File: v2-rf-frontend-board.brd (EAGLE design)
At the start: 89.7 x 43.9 mm, 134 parts, among them J1 1.27MM-SWD-CONNECTOR, J3 ROCKETNET-CONNECTOR-16M, Q1 NTR4101P, T1 ALT4532, T2 ALT4532, U1 MAX2769, U10 LMZ12001, U3 LAN8710A-EZC, U4 7Q-16.368MBG-T, U5 XC2401, U6 MAX8510EXK29+T, U7 MAX8510EXK29+T, U8 STM32F4V, X1 25 MHz, X2 BU-SMA-H

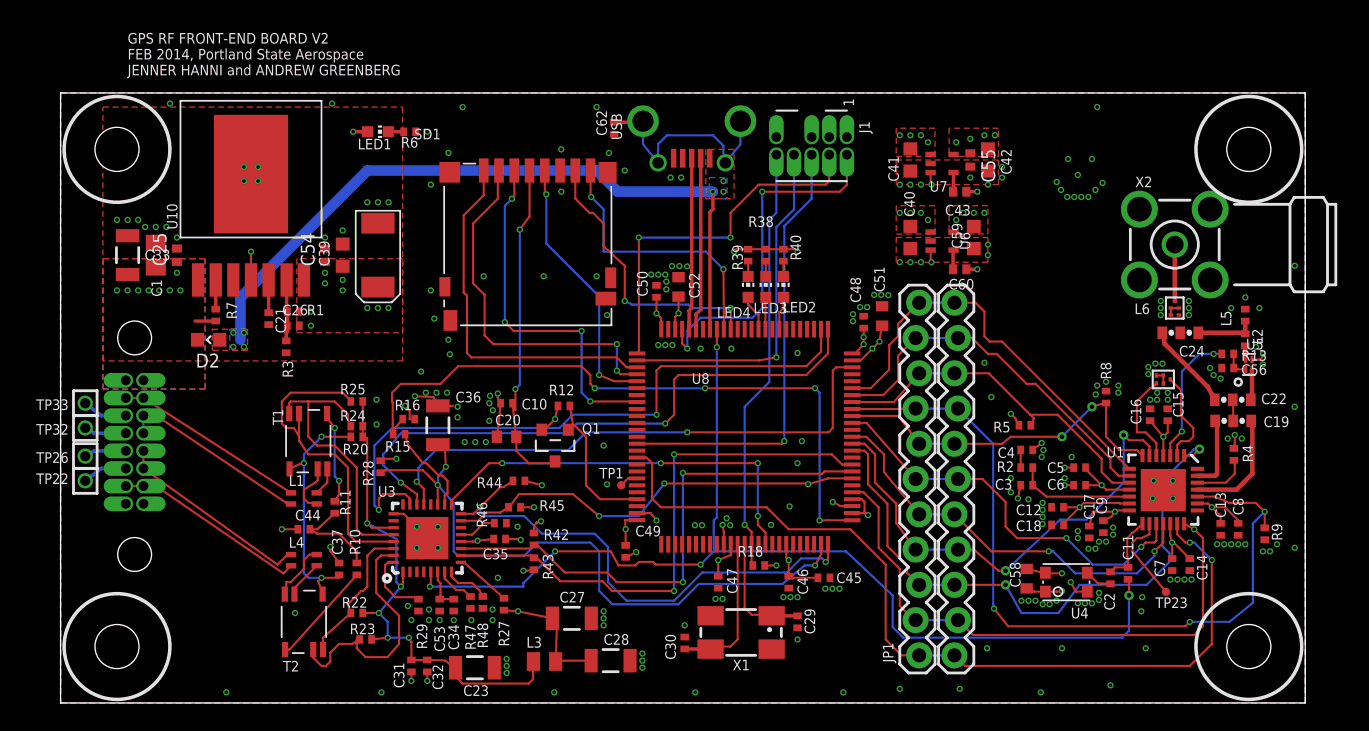
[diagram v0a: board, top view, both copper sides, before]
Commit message: Beeeeg changes to GPS board. Caught many small mistakes in STM and LAN wiring and footprints, fixed. Better layout of magnetics, replumbed the lines between STM32 and LAN, and more. Passes ERC and DRC, although still not quite done: want to double check SAW filters, find a smaller 50 MHz clock, and add other GPS interface.
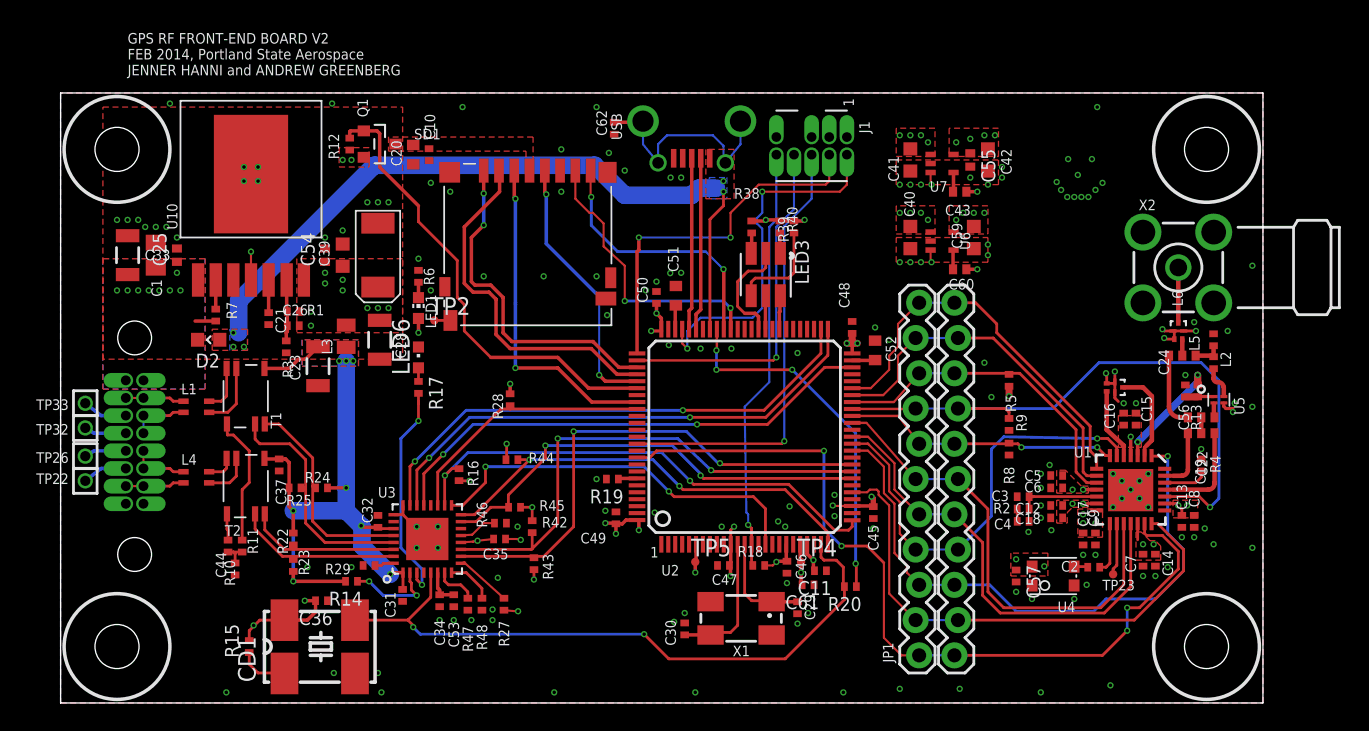
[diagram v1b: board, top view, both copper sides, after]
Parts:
- removed C27: 22uF/6.3V, rcl_custom:1206-C
- removed C58: 470nF 10V, rcl_custom:0603-C-NOSILK
- removed LED2: BLUE, led:CHIP-LED0603
- removed LED4: RED, led:CHIP-LED0603
- removed TP1: (no value), testpad:TP06R
- added C57: 470n, rcl_custom:0402-C-NOSILK
- added C61: 100n, rcl_custom:0402-C-NOSILK
- added CD1: 6NC2_CLOCK_DRIVER, gogo:7X5MM_CLOCK_DRIVER
- added LED6: (no value), led:CHIPLED_0603
- added R14, R19: 10k, rcl_custom:0402-C-NOSILK
- added R17: 1k, rcl_custom:0402-C-NOSILK
- added TP2, TP4, TP5: (no value), testpad:TP06R
- C1: value 1uF 50V -> 1u 50V
- C11: value DNP -> 100n
- C12, C14, C16, C17, C19, C22, C24, C6, C8: value 100pF 10V -> 100p
- C13, C15, C18, C45, C46, C47, C48, C49, C5, C50, C7, C9: value 100nF 10V -> 100n
- C21: value 220nF 10V -> 220n
- C23, C28: value 22uF/6.3V -> 22u
- C25: value 100n -> 100n 50V
- C29, C30: value 18pF 10V -> 10p
- C3: value 27pF 10V -> 27p
- C31, C32, C35: value 100nF 10V -> 10n
- C33: value 10uF 50V -> 10u 50V
- C34: value 100nF 10V -> 470p
- C36: value 10uF/6.3V -> 100n; device rcl_custom:1206-C -> rcl_custom:0402-C-NOSILK
- C37: value 100nF 10V -> 22n
- C4: value 470pF 10V -> 470p
- C44: value 1nF 10V -> 100n
- C51, C52: value 2.2uF 10V -> 2.2u
- C53: value 100nF 10V -> 2.2u
- C56: value 10nF 10V -> 10n
- C62: value 100n 10V -> 100n 50V
- LED3: value GREEN -> (none); device led:CHIP-LED0603 -> apdm:PLCC-6
- R10, R11: value 75 -> 50
- R15: value 150 -> 47k
- R20: value 0R -> NP
- R22, R23, R24, R25: value 49.9R/1% -> 49.9 1%
- R27, R42, R43, R44, R45, R46, R47, R48: value 4.7k -> 10k
- R29: value 12.1k/1% -> 12.1k
- U2: value STM32F4V -> STM32F4V_100PIN_GPSBOARD
- moved R20 37.2 mm to (56.9, 8.38), turned to 180 degrees
- moved C28 28.5 mm to (23.0, 26.2), turned to 90 degrees
- moved L3 27.4 mm to (20.6, 26.4), turned to 90 degrees
- moved Q1 25.1 mm to (23.0, 40.3), turned to 270 degrees
- moved C23 24.5 mm to (18.5, 24.3), turned to 90 degrees
- moved R12 24.4 mm to (20.8, 40.3), turned to 270 degrees
- moved C11 22.2 mm to (54.7, 9.53), turned to 180 degrees
- moved C20 21.4 mm to (25.4, 39.5), turned to 90 degrees
- moved R9 20.0 mm to (68.3, 20.1)
- moved C10 18.8 mm to (26.5, 39.5), turned to 90 degrees
- moved R15 18.7 mm to (13.6, 4.06), turned to 90 degrees
- moved C36 15.2 mm to (18.8, 7.37), turned to 180 degrees
- moved C51 14.9 mm to (44.3, 29.3)
- moved C52 14.9 mm to (58.7, 25.4)
- moved LED1 13.0 mm to (25.8, 28.4), turned to 0 degrees
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- renumbered U8 to U2
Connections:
- net VDD renamed SD-VDD
- removed net ETH_CRX_DV: R45.2, U2.PA7, U3.15
- removed net LED3: LED3.A, U2.PD13
- removed net LED4: LED4.A, U2.PD14
- removed net N$56: C37.2, R20.1, T1.3, T2.3
- removed net N$63: R15.2, U3.18
- removed net PHY_CLK_25MHZ: C11.1, U2.PA8, U3.5
- new net ETH_CRS_DV: R45.2, U2.32, U3.15
- new net ETH_RMII_REF_CLK: CD1.3, R20.2, U2.24, U3.5
- new net MCO1-ETH-CLK: R20.1, U2.67
- new net N$1: R14.1, U3.2
- new net N$23: LED6.A, R17.1
- new net N$24: R17.2, U3.3
- new net N$34: LED3.5, U2.60
- new net N$37: LED3.1, R40.2
- new net N$38: SD1.S1, TP2.TP
- new net N$39: CD1.1, R15.1
- new net N$43: C52.2, U2.49
- new net N$45: C51.2, U2.73
- net !RST: now also U2.14; no longer U2.NRST
- net 2.85VD: now also C57.1; no longer C58.1
- net 3.3VD: now also C11.2, C36.2, C61.2, CD1.4, R15.2, TP4.TP, TP5.TP, U2.100, U2.11, U2.19, U2.21, U2.22, U2.28, U2.50, U2.6, U2.75; no longer C27.2, C51.2, C52.2, U2.VCAP1, U2.VCAP2, U2.VDD1, U2.VDD2, U2.VDD3, U2.VDD4, U2.VDD5, U2.VDD6
- net ANTFLAG: now also U2.36; no longer U2.PB1
- net EPHY_NRST: now also U2.84; no longer C36.2, U2.PA1
- net ETH_MDC: now also U2.16; no longer U2.PC1
- net ETH_MDINT: now also U2.26, U3.18; no longer R15.1, U2.PA3
- net ETH_MDIO: now also U2.25; no longer U2.PA2
- net ETH_RXD0: now also U2.33; no longer U2.PC4
- net ETH_RXD1: now also U2.34; no longer U2.PC5
- net ETH_TXD0: now also U2.51; no longer U2.PB12
- net ETH_TXD1: now also U2.52; no longer U2.PB13
- net ETH_TX_EN: now also U2.48; no longer U2.PB11
- net GND: now also C11.1, C57.2, C61.1, CD1.2, L6.B, L6.C, L6.E, L7.B, L7.C, L7.E, LED6.C, R19.2, U2.10, U2.20, U2.27, U2.74, U2.99; no longer C27.1, C58.2, L6.2, L6.3, L6.5, L7.2, L7.3, L7.5, SD1.S1, U2.PA4, U2.PDR_ON, U2.VSS1, U2.VSS2, U2.VSS3
- net I0-DATA_OUT: now also U2.91; no longer U2.PB5
- net I1-CLK_SER: now also U2.30; no longer U2.PA5
- net LD: now also U2.37; no longer U2.PB2
- net LED2: now also LED3.2, U2.61; no longer LED2.A, U2.PD11
- net LNA2: now also L6.A; no longer L6.1
- net LNAOUT: now also L7.A; no longer L7.1
- net MAX_!IDLE: now also U2.42; no longer U2.PE11
- net MAX_!SHDN: now also U2.41; no longer U2.PE10
- net MAX_CFG_!CS: now also U2.43; no longer U2.PE12
- net MAX_CFG_MOSI: now also U2.45; no longer U2.PE14
- net MAX_CFG_SCLK: now also U2.44; no longer U2.PE13
- net MIXIN: now also L7.D; no longer L7.4
- net N$11: now also LED3.6, U2.58; no longer LED2.C, R40.2
- net N$12: now also LED3.4, R39.2; no longer LED3.C, R38.2
- net N$18: now also LED3.3, R38.2; no longer LED4.C, R39.2
- net N$21: now also L6.D; no longer L6.4
- net N$9: now also R19.1, U2.94; no longer TP1.TP, U2.BOOT0
- net OSC_IN: now also U2.12; no longer U2.PH0
- net OSC_OUT: now also U2.13; no longer U2.PH1
- net OTG_FS_DM: now also U2.70; no longer U2.PA11
- net OTG_FS_DP: now also U2.71; no longer U2.PA12
- net OTG_FS_VBUS: now also U2.68; no longer U2.PA9
- net PE0: now also U2.81; no longer U2.PE0
- net Q0-DATASYNC: now also U2.38; no longer U2.PE7
- net Q1-TIMESYNC: now also U2.40; no longer U2.PE9
- net SDIO_CLK: now also U2.80; no longer U2.PC12
- net SDIO_CMD: now also U2.83; no longer U2.PD2
- net SDIO_D0: now also U2.65; no longer U2.PC8
- net SDIO_D1: now also U2.66; no longer U2.PC9
- net SDIO_D2: now also U2.78; no longer U2.PC10
- net SDIO_D3: now also U2.79; no longer U2.PC11
- net TCK: now also U2.76; no longer U2.PA14
- net TDI: now also U2.77; no longer U2.PA15
- net TDO: now also U2.89; no longer U2.PB3
- net TMS: now also U2.72; no longer U2.PA13
- net VDDA: now also C37.2, R14.2, T1.3, T2.3; no longer R20.2
- net XTAL: no longer C11.2
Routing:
- net PHY_CLK_25MHZ: track 77.7 -> 0.00 mm, vias 5 -> 0
- net ETH_RMII_REF_CLK: track 0.00 -> 47.6 mm, vias 0 -> 2
- net ETH_CRS_DV: track 0.00 -> 32.6 mm, vias 0 -> 2
- net ETH_CRX_DV: track 31.0 -> 0.00 mm, vias 3 -> 0
- net EPHY_NRST: track 47.6 -> 18.9 mm, vias 3 -> 0
- net MCO1-ETH-CLK: track 0.00 -> 25.9 mm, vias 0 -> 4
- net SD-VDD: track 24.8 -> 0.00 mm, vias 2 -> 0
- net PE0: track 10.7 -> 33.6 mm
- net GND: track 35.7 -> 15.0 mm, vias 257 -> 156
- net N$56: track 17.9 -> 0.00 mm, vias 3 -> 0
- net N$24: track 0.00 -> 16.0 mm, vias 0 -> 2
- net 2.85VA: track 21.8 -> 6.06 mm, vias 9 -> 12
- net ETH_MDINT: track 48.4 -> 36.3 mm, vias 4 -> 2
- net MAX_!IDLE: track 57.3 -> 46.1 mm, vias 3 -> 1
- net 2.85VD: track 13.5 -> 2.92 mm, vias 9 -> 13
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- added copper zone on layer 1, net SD-VDD
- added copper zone on layer 1, net VDDA
- added copper zone on layer 16, net VDDA
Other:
- board size 89.7 x 43.9 mm -> 86.6 x 43.9 mm
